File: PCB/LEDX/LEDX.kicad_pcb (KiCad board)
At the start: 2 copper layers, 70 x 70 mm, 25 parts, among them J2 Conn_01x03, J3 TC2030-USB-NL-DS, U1 ICS43434_MEMS_Mic, U2 ESP32-S3-MINI-1, U3 78L05, U5 MD8942

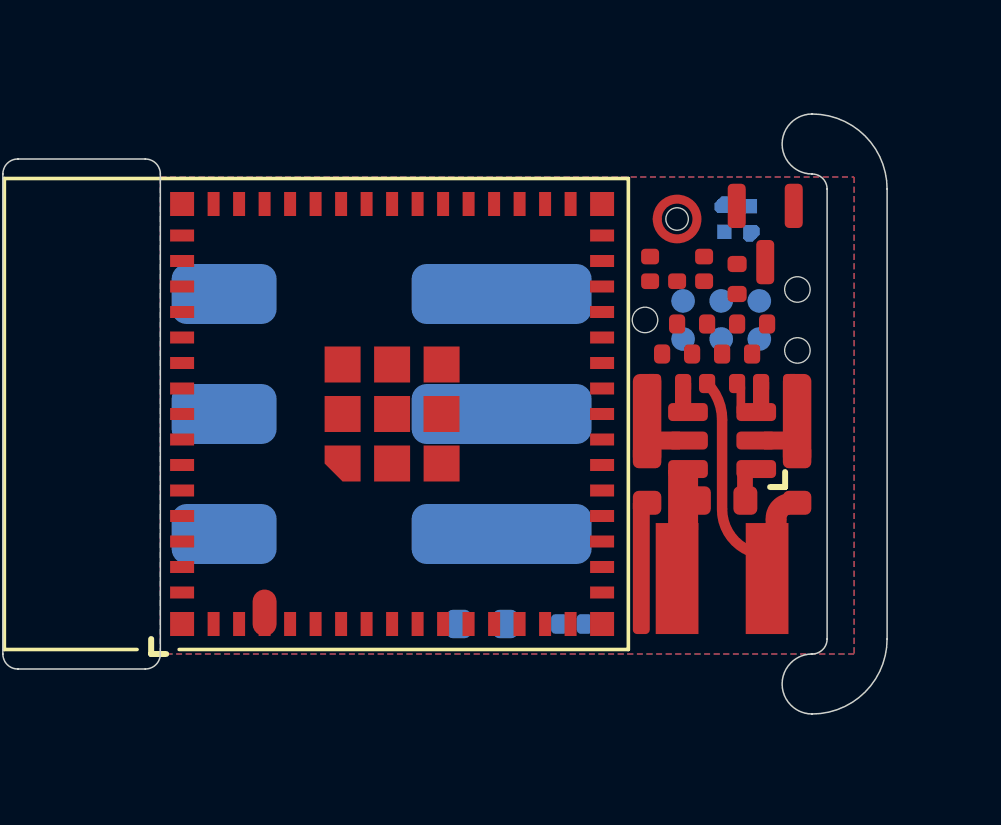
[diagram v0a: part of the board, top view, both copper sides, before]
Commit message: Tracked
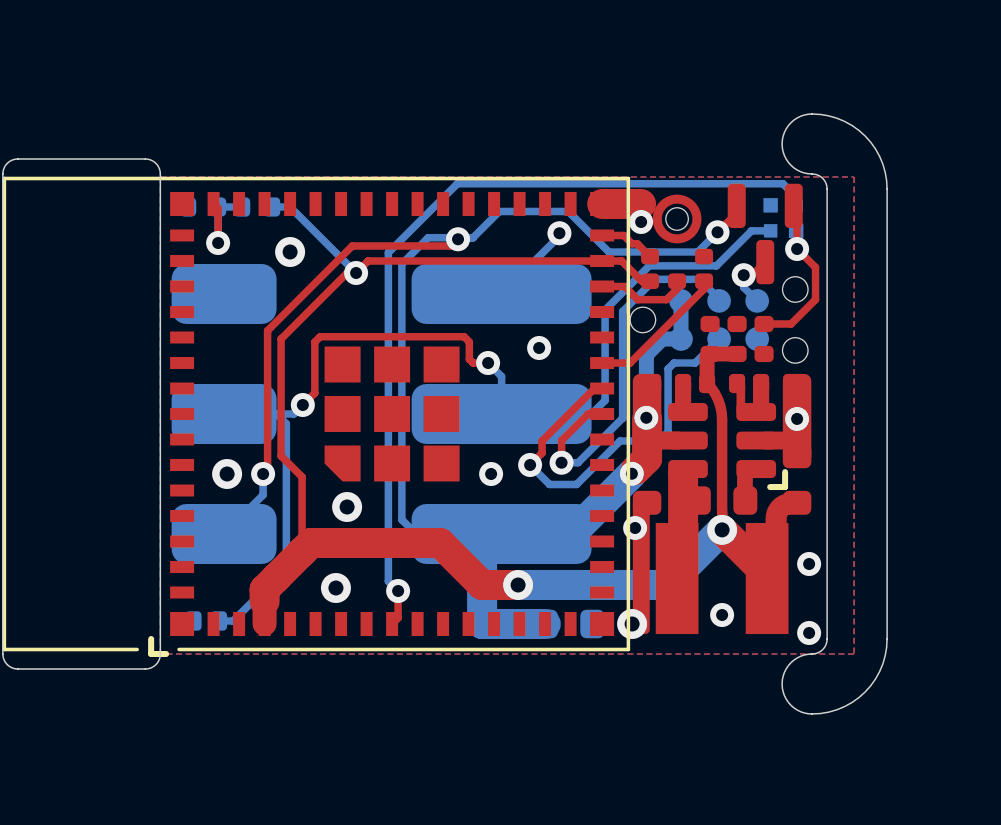
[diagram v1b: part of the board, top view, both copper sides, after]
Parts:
- C3, R1: moved to B.Cu
- moved C3 18.7 mm to (93.7, 93.1)
- moved R1 16.7 mm to (95.5, 93.1), turned to 180 degrees
- moved D2 12.2 mm to (93.8, 106.9)
- moved C4 2.90 mm to (105.9, 107.0), turned to 0 degrees
- moved C5 2.19 mm to (112.4, 97.5)
- moved C1 1.58 mm to (111.5, 97.5), turned to 90 degrees
- moved D1 1.54 mm to (113.0, 93.5), turned to 0 degrees
- moved C2 1.21 mm to (110.6, 97.5), turned to 90 degrees
- moved J3 0.07 mm to (110.9, 96.9)
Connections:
- U2 pad 16: WS -> unconnected-(U2-GPIO12-Pad16)
- U2 pad 17: SD -> unconnected-(U2-GPIO13-Pad17)
- U2 pad 18: +3.3V -> unconnected-(U2-GPIO14-Pad18)
- U2 pad 19: SCK -> unconnected-(U2-GPIO15-Pad19)
- U2 pad 25: unconnected-(U2-GPIO21-Pad25) -> WS
- U2 pad 28: unconnected-(U2-GPIO33-Pad28) -> SD
- U2 pad 29: unconnected-(U2-GPIO34-Pad29) -> +3.3V
- U2 pad 30: unconnected-(U2-GPIO48-Pad30) -> SCK
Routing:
- net DC: track 0.00 -> 53.5 mm, vias 0 -> 5
- net +3.3V: track 0.75 -> 47.2 mm, vias 0 -> 3
- net Net-(D1-O): track 0.00 -> 36.7 mm, vias 0 -> 2
- net LED: track 0.00 -> 27.6 mm, vias 0 -> 1
- net D+: track 0.00 -> 13.2 mm, vias 0 -> 1
- net D-: track 0.00 -> 12.7 mm, vias 0 -> 1
- net GND: track 0.00 -> 7.61 mm, vias 0 -> 15
- net Net-(D1-+): track 0.00 -> 5.94 mm, vias 0 -> 1
- net WS: track 0.00 -> 4.68 mm
- net Net-(U2-EN): track 0.00 -> 3.36 mm, vias 0 -> 1
- net SD: track 0.00 -> 3.09 mm
- net SCK: track 0.00 -> 1.89 mm
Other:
- board text added: "led.revk.uk"
